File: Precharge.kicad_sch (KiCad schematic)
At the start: 16 parts, among them J1 BMS_Sig, J2 JST-XA, J3 MicroFit+, J4 JST-XA, K1 DAR71205, K2 Relay_SPDT_G6RN, Q1 BSS205N, Q2 BSS205N

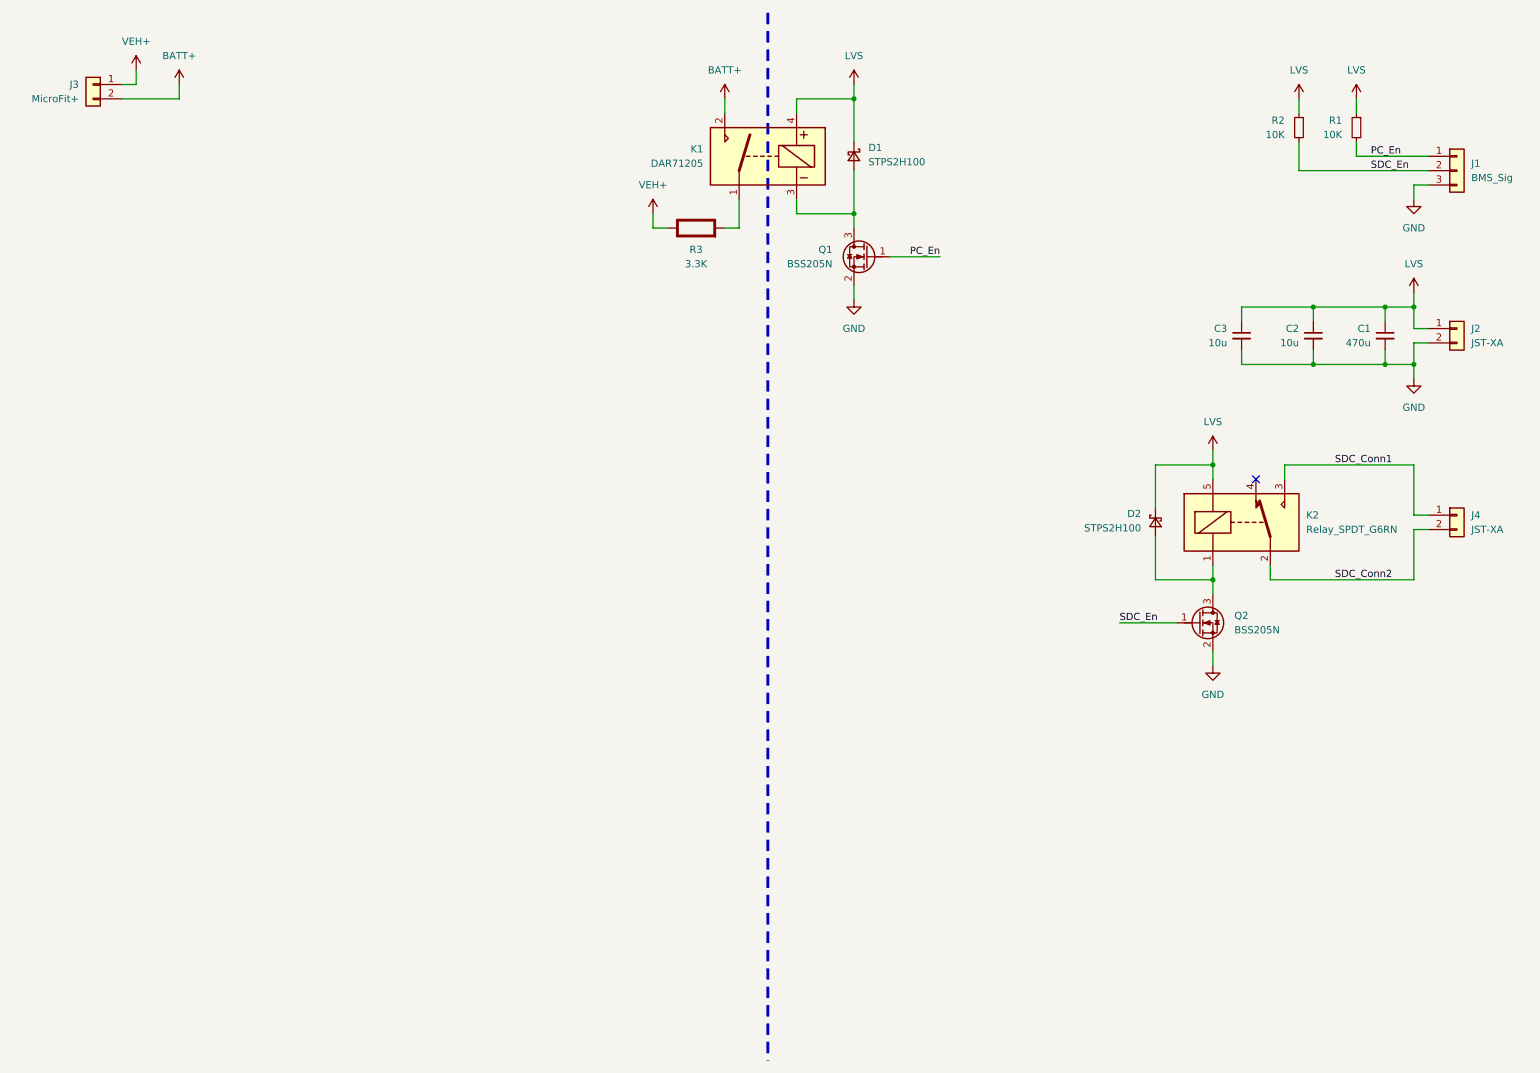
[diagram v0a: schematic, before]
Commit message: Finished schematic and PCB
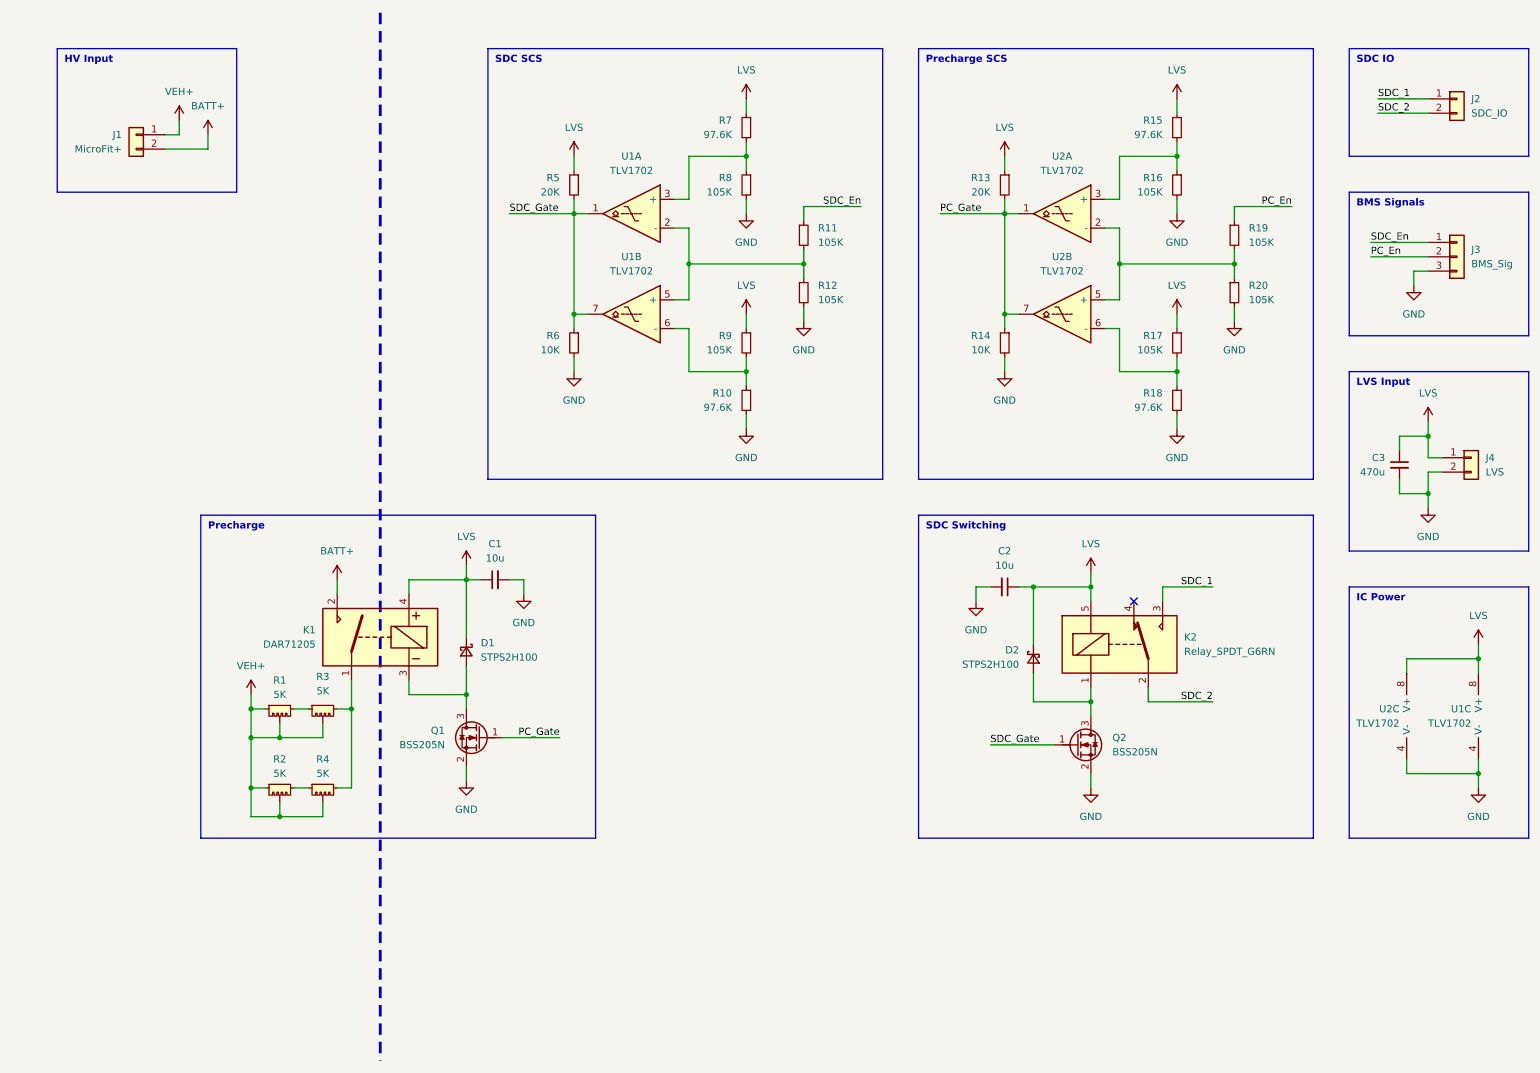
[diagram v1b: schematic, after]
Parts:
- removed C3: 10u, Capacitor_SMD:C_1206_3216Metric_Pad1.33x1.80mm_HandSolder, symbol Device:C_Small
- removed R1, R2: 10K, Resistor_SMD:R_0805_2012Metric_Pad1.20x1.40mm_HandSolder, symbol Device:R_Small
- removed R3: 3.3K, customFootprints:HS100, symbol PCM_Elektuur:R
- added C1: 10u, Capacitor_SMD:C_1206_3216Metric_Pad1.33x1.80mm_HandSolder, symbol Device:C_Small
- added R1, R2, R3, R4: 5K, Package_TO_SOT_SMD:TO-263-2, symbol customSymbols:R_HS
- added R10, R15, R18, R7: 97.6K, Resistor_SMD:R_0805_2012Metric_Pad1.20x1.40mm_HandSolder, symbol Device:R_Small
- added R11, R12, R16, R17, R19, R20, R8, R9: 105K, Resistor_SMD:R_0805_2012Metric_Pad1.20x1.40mm_HandSolder, symbol Device:R_Small
- added R13, R5: 20K, Resistor_SMD:R_0805_2012Metric_Pad1.20x1.40mm_HandSolder, symbol Device:R_Small
- added R14, R6: 10K, Resistor_SMD:R_0805_2012Metric_Pad1.20x1.40mm_HandSolder, symbol Device:R_Small
- added U1, U2: TLV1702, Custom_MSM:Comparator_Dual_VSSOP-8, symbol Custom_MSM:Comparator_Dual_Open-Coll
- J2: renamed from J4; value JST-XA -> SDC_IO
- J4: renamed from J2; value JST-XA -> LVS; S1PC (none) -> 0.30; S2PC (none) -> 0.36
- renumbered C1 to C3, J3 to J1, J1 to J3
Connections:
- net GND: now also C1.2, R10.2, R12.2, R14.2, R16.2, R18.2, R20.2, R6.2, R8.2, U1.4 (V-), U2.4 (V-)
- net LVS: now also C1.1, R13.1, R15.1, R17.1, R5.1, R7.1, R9.1, U1.8 (V+), U2.8 (V+)
- net PC_En: now also J3.2 (Pin_2), R19.1; no longer J3.1 (Pin_1), Q1.1 (G)
- net SDC_En: now also J3.1 (Pin_1), R11.1; no longer J3.2 (Pin_2), Q2.1 (G)
- net VEH+: now also R1.1, R1.2, R2.1, R2.2, R3.2, R4.2
- net at K1.1: now also R3.3, R4.3
- net SDC_Conn1 renamed SDC_1
- net SDC_Conn2 renamed SDC_2
- new net: R11.2, R12.1, U1.2 (-), U1.5 (+)
- new net: R1.3, R3.1
- new net: R17.2, R18.1, U2.6 (-)
- new net: R10.1, R9.2, U1.6 (-)
- new net: R19.2, R20.1, U2.2 (-), U2.5 (+)
- new net: R15.2, R16.1, U2.3 (+)
- new net: R7.2, R8.1, U1.3 (+)
- new net: R2.3, R4.1
- new net PC_Gate: Q1.1 (G), R13.2, R14.1, U2.1, U2.7
- new net SDC_Gate: Q2.1 (G), R5.2, R6.1, U1.1, U1.7
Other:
- note added: "BMS Signals"
- note added: "HV Input"
- note added: "IC Power"
- note added: "LVS Input"
- note added: "Precharge"
- note added: "Precharge SCS"
- note added: "SDC IO"
- note added: "SDC SCS"
- note added: "SDC Switching"
- moved on the sheet: C3, D1, D2, J1, J2, J3, J4, K1, K2, Q1, Q2
